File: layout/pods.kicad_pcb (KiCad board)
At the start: 2 copper layers, 38.1 x 82.6 mm, 17 parts, among them J1 BATTERY, SW2 A, SW3 POWER, U1 STM32F103RCT6, U2 nRF24L01+, U3 MT-02, U4 ADP1710AUJZ, U5 SWD, U6 TP4056, U7 SH1106

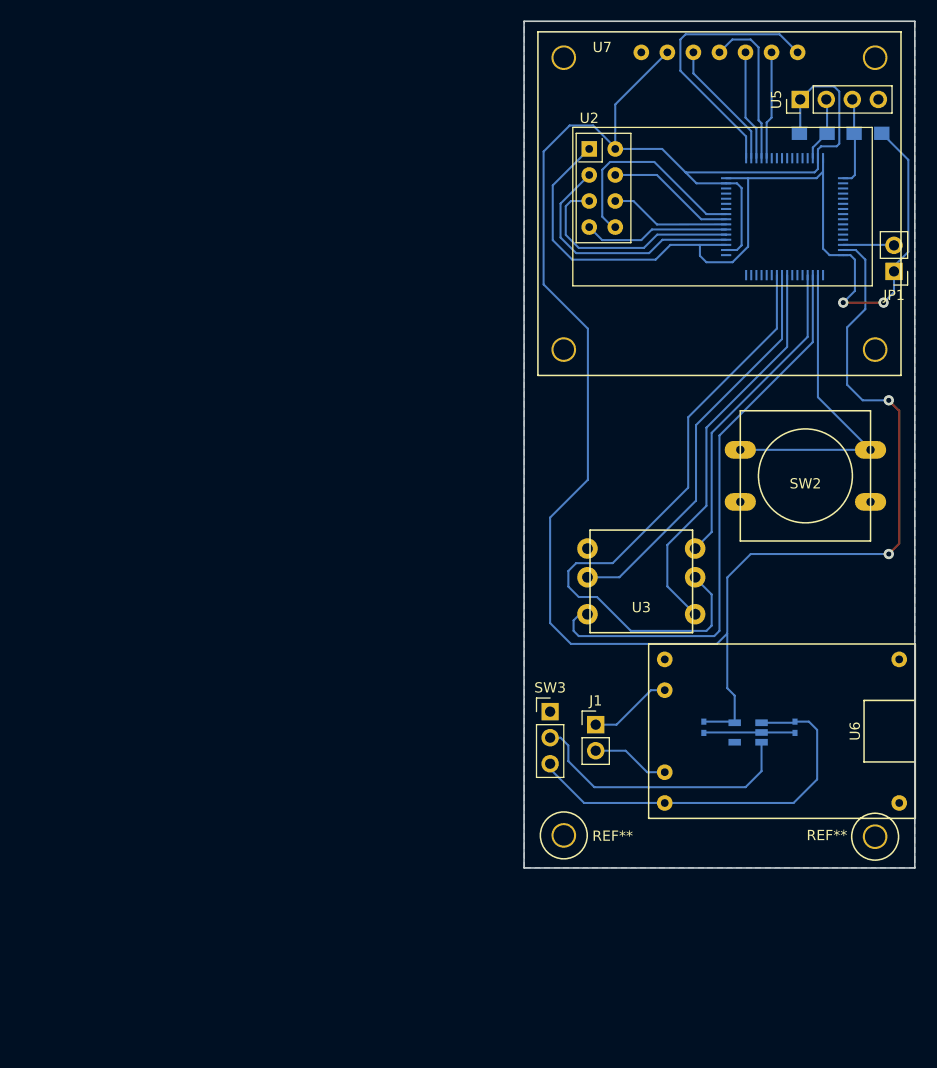
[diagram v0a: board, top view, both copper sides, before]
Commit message: New PCB design
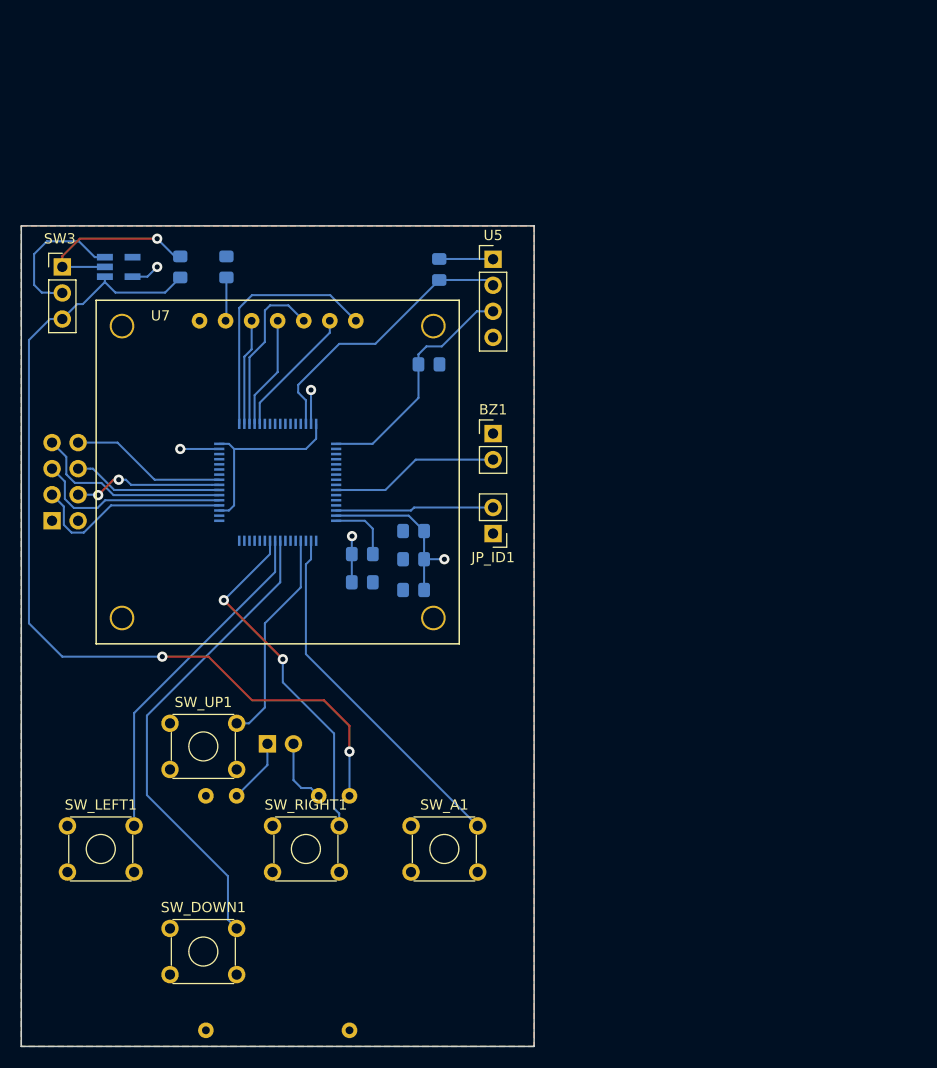
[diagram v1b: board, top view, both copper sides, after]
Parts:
- removed JP1: Jumper, Pin_Headers:Pin_Header_Straight_1x02_Pitch2.54mm
- removed REF** (x2): 1pin, Connectors:1pin
- removed SW2: A, Buttons_Switches_THT:SW_PUSH-12mm
- removed U3: MT-02, mt02:MT-02
- added BZ1: Buzzer, Connector_PinHeader_2.54mm:PinHeader_1x02_P2.54mm_Vertical, F.Cu at (119.7, 64.7)
- added C3: 100n, Capacitor_SMD:C_0805_2012Metric_Pad1.15x1.40mm_HandSolder, B.Cu at (106.9, 79.2)
- added C4: 100n, Capacitor_SMD:C_0805_2012Metric_Pad1.15x1.40mm_HandSolder, B.Cu at (106.9, 76.5)
- added C5: 100n, Capacitor_SMD:C_0805_2012Metric_Pad1.15x1.40mm_HandSolder, B.Cu at (111.9, 80.0)
- added C6: 100n, Capacitor_SMD:C_0805_2012Metric_Pad1.15x1.40mm_HandSolder, B.Cu at (111.9, 77.0)
- added C7: 100n, Capacitor_SMD:C_0805_2012Metric_Pad1.15x1.40mm_HandSolder, B.Cu at (111.9, 74.2)
- added JP_ID1: Jumper, Connector_PinHeader_2.54mm:PinHeader_1x02_P2.54mm_Vertical, F.Cu at (119.7, 74.5)
- added SW_A1: A, Button_Switch_THT:SW_TH_Tactile_Omron_B3F-10xx, F.Cu at (111.7, 103.0)
- added SW_DOWN1: A, Button_Switch_THT:SW_TH_Tactile_Omron_B3F-10xx, F.Cu at (88.2, 113.0)
- added SW_LEFT1: A, Button_Switch_THT:SW_TH_Tactile_Omron_B3F-10xx, F.Cu at (78.2, 103.0)
- added SW_RIGHT1: A, Button_Switch_THT:SW_TH_Tactile_Omron_B3F-10xx, F.Cu at (98.2, 103.0)
- added SW_UP1: A, Button_Switch_THT:SW_TH_Tactile_Omron_B3F-10xx, F.Cu at (88.2, 93.0)
- C1, C2: footprint Capacitors_SMD:C_0402_NoSilk -> Capacitor_SMD:C_0805_2012Metric_Pad1.15x1.40mm_HandSolder
- J1: footprint Pin_Headers:Pin_Header_Straight_1x02_Pitch2.54mm -> Connector_PinHeader_2.54mm:PinHeader_1x02_P2.54mm_Vertical; moved to B.Cu
- R1, R2: footprint Resistors_SMD:R_0805_HandSoldering -> Resistor_SMD:R_0805_2012Metric_Pad1.15x1.40mm_HandSolder
- SW3: footprint Pin_Headers:Pin_Header_Straight_1x03_Pitch2.54mm -> Connector_PinHeader_2.54mm:PinHeader_1x03_P2.54mm_Vertical
- U2: footprint RF_Modules:nRF24L01_Breakout -> Connector_PinHeader_2.54mm:PinHeader_2x04_P2.54mm_Vertical; moved to B.Cu
- U4: value ADP1710AUJZ -> ADP; footprint TO_SOT_Packages_SMD:TSOT-23-5 -> Package_TO_SOT_SMD:SOT-23-5_HandSoldering
- U5: footprint Pin_Headers:Pin_Header_Straight_1x04_Pitch2.54mm -> Connector_PinHeader_2.54mm:PinHeader_1x04_P2.54mm_Vertical
- U6: footprint tp4056 -> tp4056:tp4056; moved to B.Cu
- moved U4 76.3 mm to (83.2, 48.5), turned to 0 degrees
- moved C1 74.9 mm to (89.2, 48.5), turned to 90 degrees
- moved C2 64.7 mm to (93.7, 48.5), turned to 90 degrees
- moved SW3 64.4 mm to (77.7, 48.5)
- moved U2 63.7 mm to (76.7, 73.2)
- moved U1 55.8 mm to (98.7, 69.5)
- moved U6 52.3 mm to (98.7, 111.5), turned to 0 degrees
- moved U7 50.4 mm to (98.7, 68.5)
- moved R2 48.4 mm to (113.4, 58.0)
- moved R1 38.8 mm to (114.4, 48.7), turned to 90 degrees
- moved U5 33.8 mm to (119.7, 47.7), turned to 0 degrees
- moved J1 32.1 mm to (97.7, 95.0), turned to 270 degrees
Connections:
- U1 pad 1: Net-(U1-Pad1) -> (no net)
- U1 pad 11: Net-(U1-Pad11) -> (no net)
- U1 pad 12: Net-(U1-Pad12) -> (no net)
- U1 pad 13: Net-(U1-Pad13) -> (no net)
- U1 pad 14: Net-(U1-Pad14) -> (no net)
- U1 pad 15: Net-(U1-Pad15) -> (no net)
- U1 pad 16: Net-(U1-Pad16) -> (no net)
- U1 pad 17: Net-(U1-Pad17) -> (no net)
- U1 pad 26: Net-(U1-Pad26) -> (no net)
- U1 pad 27: Net-(U1-Pad27) -> (no net)
- U1 pad 28: Net-(U1-Pad28) -> (no net)
- U1 pad 29: Net-(U1-Pad29) -> (no net)
- U1 pad 3: BUTTON_B -> (no net)
- U1 pad 30: Net-(U1-Pad30) -> (no net)
- U1 pad 38: Net-(U1-Pad38) -> (no net)
- U1 pad 39: Net-(U1-Pad39) -> (no net)
- U1 pad 40: Net-(U1-Pad40) -> (no net)
- U1 pad 41: Net-(U1-Pad41) -> (no net)
- U1 pad 42: Net-(U1-Pad42) -> (no net)
- U1 pad 43: Net-(U1-Pad43) -> (no net)
- U1 pad 44: Net-(U1-Pad44) -> (no net)
- U1 pad 45: Net-(U1-Pad45) -> (no net)
- U1 pad 5: Net-(U1-Pad5) -> (no net)
- U1 pad 50: Net-(U1-Pad50) -> (no net)
- U1 pad 51: Net-(U1-Pad51) -> (no net)
- U1 pad 52: Net-(U1-Pad52) -> (no net)
- U1 pad 53: Net-(U1-Pad53) -> (no net)
- U1 pad 54: Net-(U1-Pad54) -> (no net)
- U1 pad 55: Net-(U1-Pad55) -> (no net)
- U1 pad 56: Net-(U1-Pad56) -> (no net)
- U1 pad 57: Net-(U1-Pad57) -> (no net)
- U1 pad 58: Net-(U1-Pad58) -> SOUND
- U1 pad 59: Net-(U1-Pad59) -> (no net)
- U1 pad 6: Net-(U1-Pad6) -> (no net)
- U1 pad 60: Net-(U1-Pad60) -> (no net)
- U1 pad 61: Net-(U1-Pad61) -> (no net)
- U1 pad 7: Net-(U1-Pad7) -> (no net)
- U4 pad 4: Net-(U4-Pad4) -> (no net)
- U6 pad 3: Net-(U6-Pad3) -> (no net)
- U6 pad 4: Net-(U6-Pad4) -> (no net)
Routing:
- net +3V3: track 210.6 -> 40.8 mm, vias 2 -> 5
- net GND: track 100.2 -> 43.2 mm, vias 2 -> 1
- net BUTTON_B: track 55.7 -> 0.00 mm
- net +4V: track 41.4 -> 88.5 mm, vias 0 -> 2
- net BUTTON_RIGHT: track 62.2 -> 34.3 mm, vias 0 -> 2
- net SWDIO: track 6.34 -> 27.6 mm
- net SOUND: track 0.00 -> 16.5 mm
- net SWCLK: track 8.76 -> 23.1 mm
- net Net-(SW3-Pad2): track 27.0 -> 14.1 mm
- net DEVICE_ID: track 4.99 -> 15.4 mm
- net BUTTON_UP: track 31.2 -> 21.1 mm
- net BUTTON_DOWN: track 39.0 -> 46.8 mm
- net BUTTON_LEFT: track 39.1 -> 33.5 mm
- net OLED_RES: track 10.8 -> 16.3 mm
- net NRF_IRQ: track 20.8 -> 15.3 mm
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- added copper zone on F.Cu, net +3V3
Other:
- board size 38.1 x 82.6 mm -> 50 x 80 mm
- board text removed: "BTN"
- board text removed: "JOYSTICK"
- board text removed: "USB"
